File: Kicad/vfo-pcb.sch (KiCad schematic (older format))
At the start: 48 parts, among them J10 Link-out 1a, J11 RxTx, J13 Link-out 1b, J14 V12, J17 Link-out 2a, J18 Link-out 3, J19 Link-out 2b, J2 Conn_01x07_Female, J3 Si5351, J4 ESP32L, J5 ESP32R, J6 Rotery Encoder1, J7 ILI9341, J8 Rotery Encoder2, J9 Analog in 3-6, SW1 Rotary_Encoder_Switch, U1 AS179-92LF, U2 74HC595, U3 L7805, U4 AS179-92LF

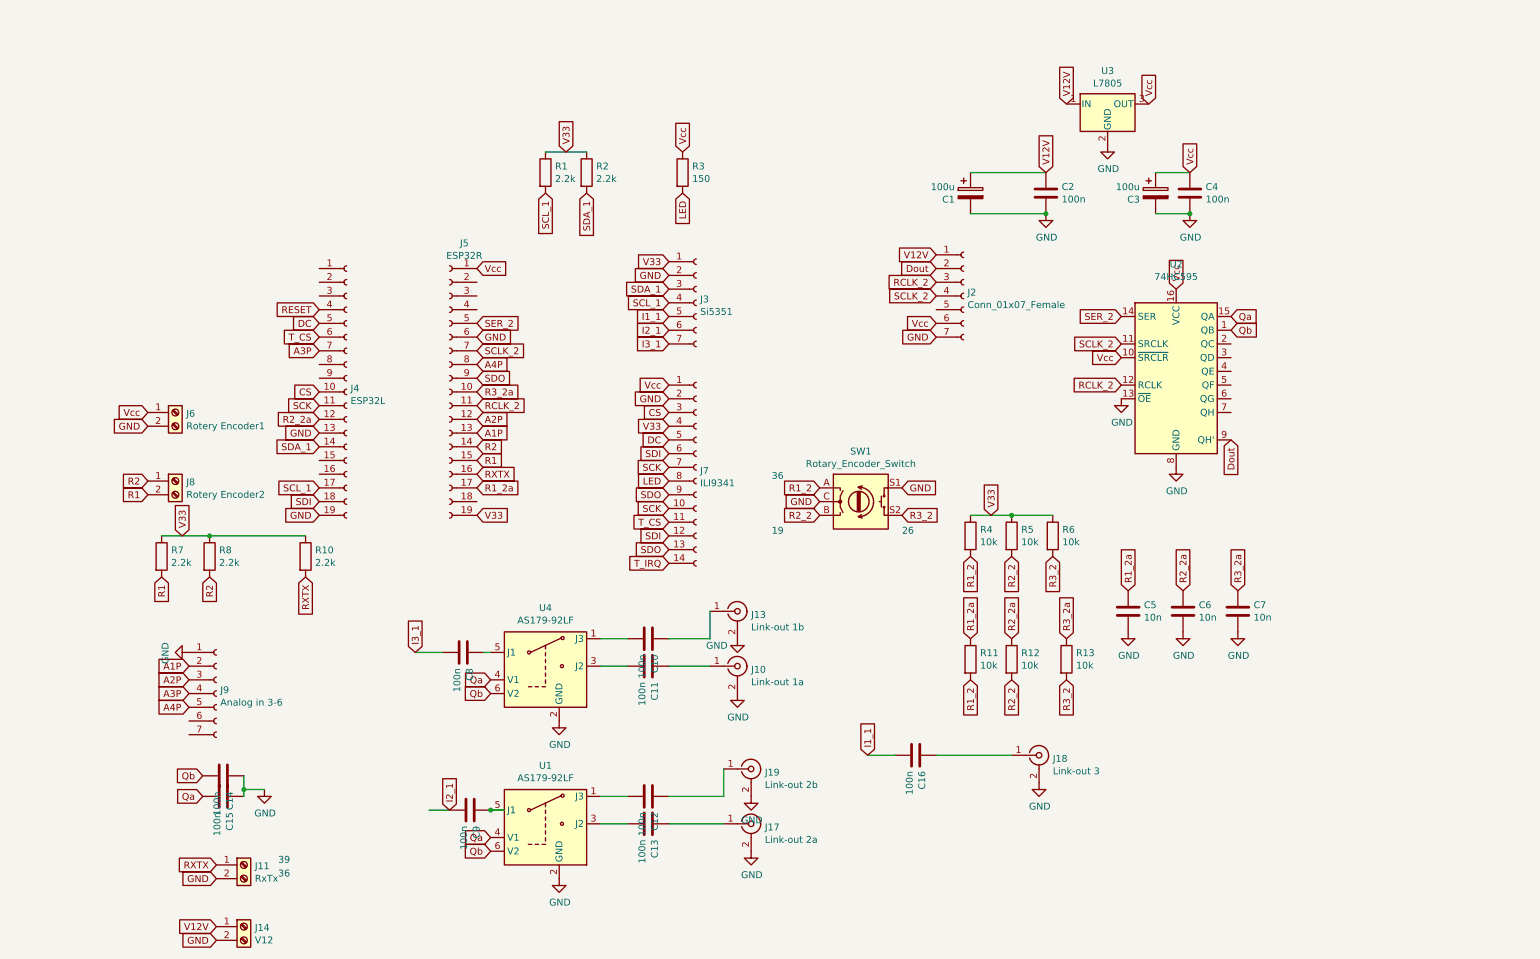
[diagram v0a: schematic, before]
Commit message: Add files via upload
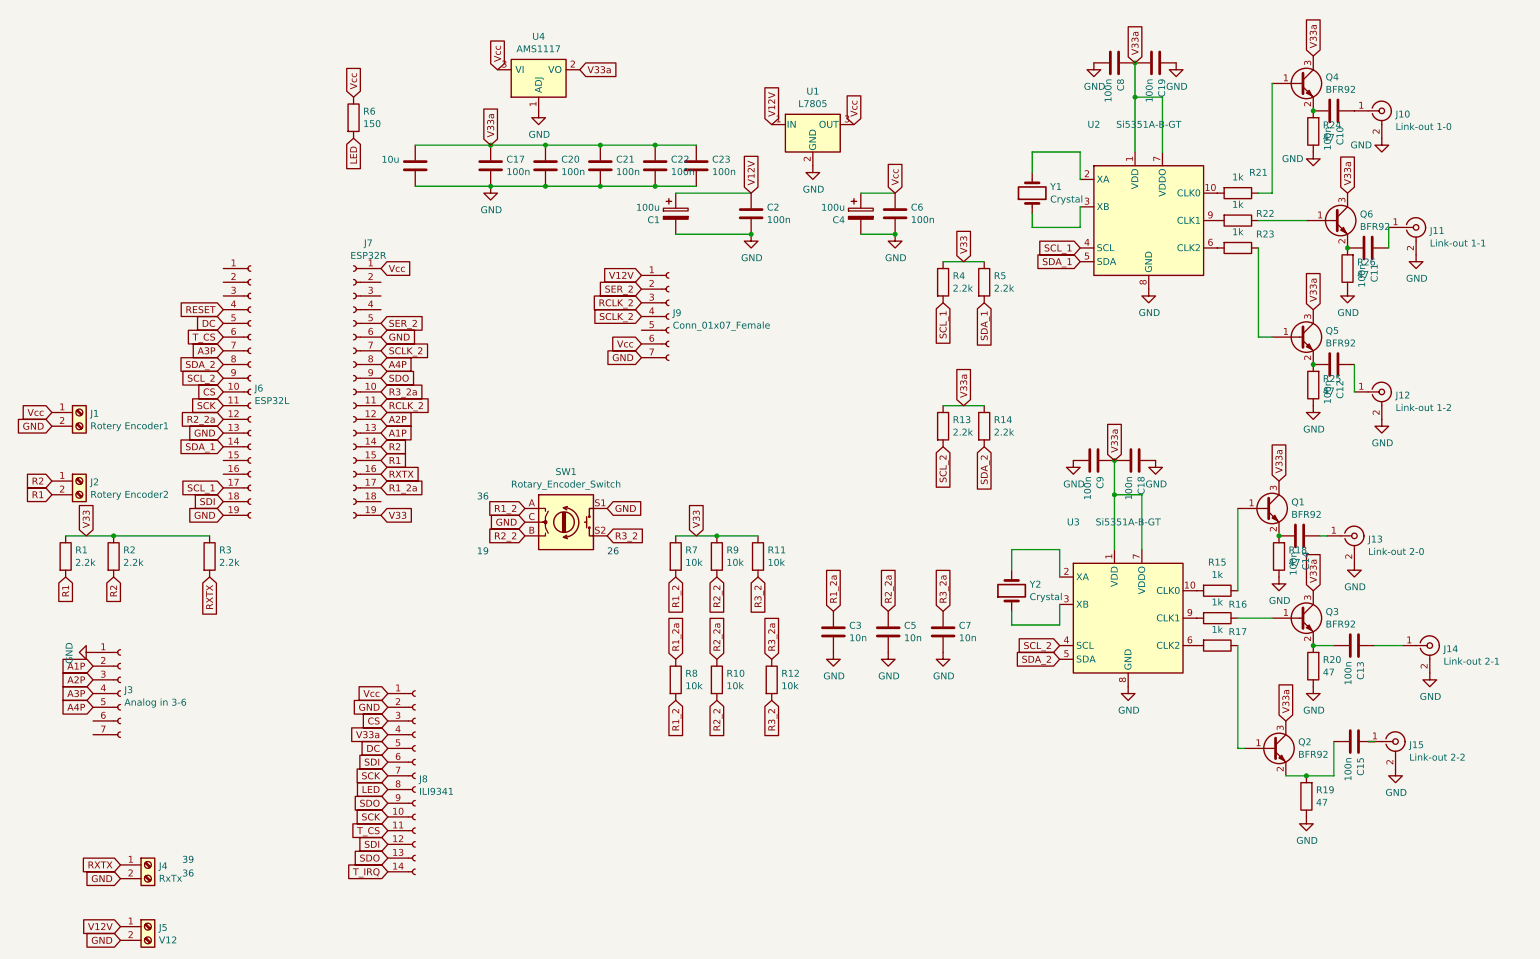
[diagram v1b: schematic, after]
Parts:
- removed J18: Link-out 3, Connector_Coaxial:SMA_Amphenol_132134_Vertical, symbol Connector:Conn_Coaxial
- removed J3: Si5351, Connector_PinSocket_2.54mm:PinSocket_1x07_P2.54mm_Vertical, symbol Connector:Conn_01x07_Female
- removed U1, U4: AS179-92LF, Package_TO_SOT_SMD:SOT-363_SC-70-6, symbol RF_Switch:AS179-92LF
- removed U2: 74HC595, Package_DIP:DIP-16_W7.62mm_LongPads, symbol 74xx:74HC595
- added C17, C18, C19, C20, C21, C22, C23: 100n, Capacitor_SMD:C_1206_3216Metric_Pad1.42x1.75mm_HandSolder, symbol Device:C
- added J12: Link-out 1-2, Connector_Coaxial:SMA_Amphenol_132134_Vertical, symbol Connector:Conn_Coaxial
- added J15: Link-out 2-2, Connector_Coaxial:SMA_Amphenol_132134_Vertical, symbol Connector:Conn_Coaxial
- added Q1, Q2, Q3, Q4, Q5, Q6: BFR92, Package_TO_SOT_SMD:SOT-323_SC-70, symbol Transistor_BJT135:BFR92
- added R13, R14: 2.2k, Resistor_SMD:R_1206_3216Metric_Pad1.42x1.75mm_HandSolder, symbol Device:R
- added R15, R16, R17, R21, R22, R23: 1k, Resistor_SMD:R_1206_3216Metric_Pad1.42x1.75mm_HandSolder, symbol Device:R
- added R18, R19, R20, R24, R25, R26: 47, Resistor_SMD:R_1206_3216Metric_Pad1.42x1.75mm_HandSolder, symbol Device:R
- added U2, U3: Si5351A-B-GT, Package_SO:MSOP-10_3x3mm_P0.5mm, symbol Oscillator:Si5351A-B-GT
- added U4: AMS1117, Package_TO_SOT_SMD:SOT-223-3_TabPin2, symbol Regulator_Linear:AMS1117
- added Y1, Y2: Crystal, Crystal:Crystal_SMD_TXC_7M-4Pin_3.2x2.5mm_HandSoldering, symbol Device:Crystal
- C16: value 100n -> 10u
- J10: renamed from J13; value Link-out 1b -> Link-out 1-0
- J11: renamed from J10; value Link-out 1a -> Link-out 1-1
- J13: renamed from J19; value Link-out 2b -> Link-out 2-0
- J14: renamed from J17; value Link-out 2a -> Link-out 2-1
- renumbered C5 to C3, C3 to C4, C6 to C5, C4 to C6, J6 to J1, J8 to J2, J9 to J3, J11 to J4, J14 to J5, J4 to J6, J5 to J7, J7 to J8, J2 to J9, R7 to R1, R12 to R10, R6 to R11, R13 to R12, R8 to R2, R10 to R3, R1 to R4, R2 to R5, R3 to R6, R4 to R7, R11 to R8, R5 to R9, U3 to U1
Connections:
- net labels added: SCL_2, SDA_2, V33a
- net labels removed: Dout, I1_1, I2_1, I3_1, Qa, Qb
- wire segments 28 -> 58
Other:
- moved on the sheet: C1, C2, C3, C4, C5, C6, C7, J1, J10, J11, J13, J14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
